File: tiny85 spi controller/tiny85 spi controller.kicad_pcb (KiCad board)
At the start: 2 copper layers, 11 parts, among them J1 rs232, J3 ISP, SW1 SW_Push, U1 MAX232, U2 ATtiny85V-10SU

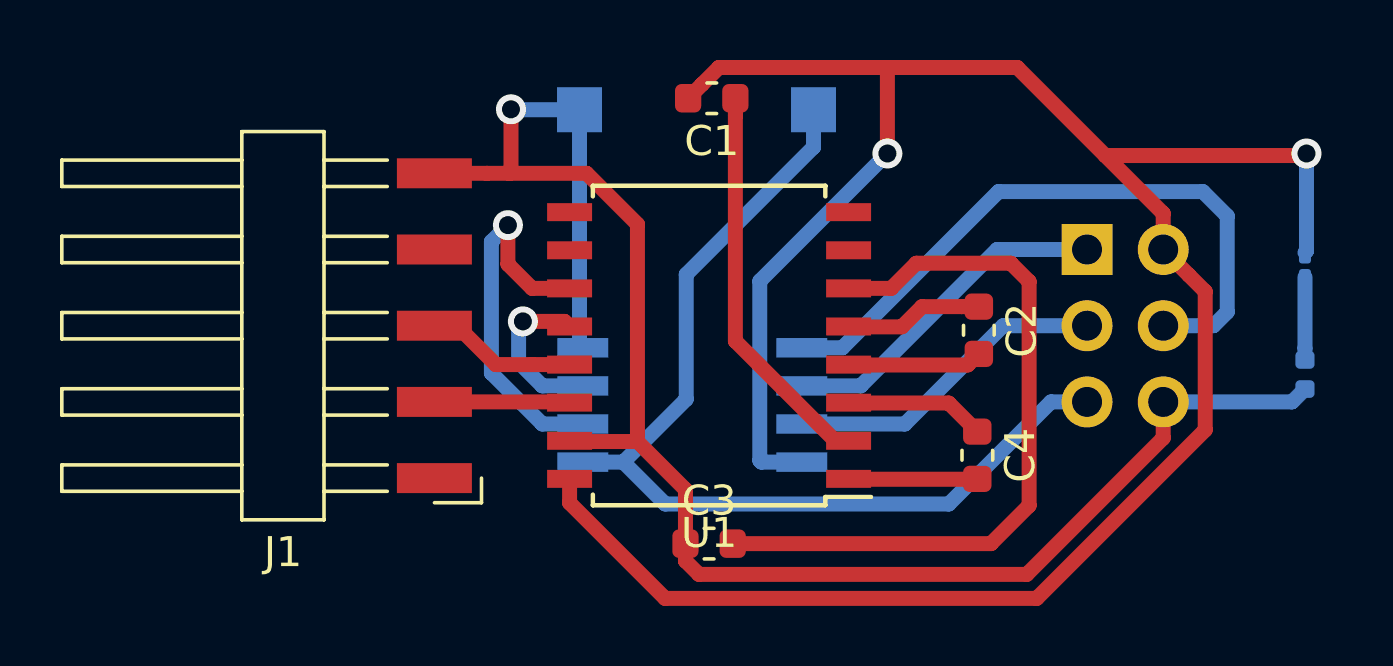
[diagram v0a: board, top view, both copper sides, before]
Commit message: some updates
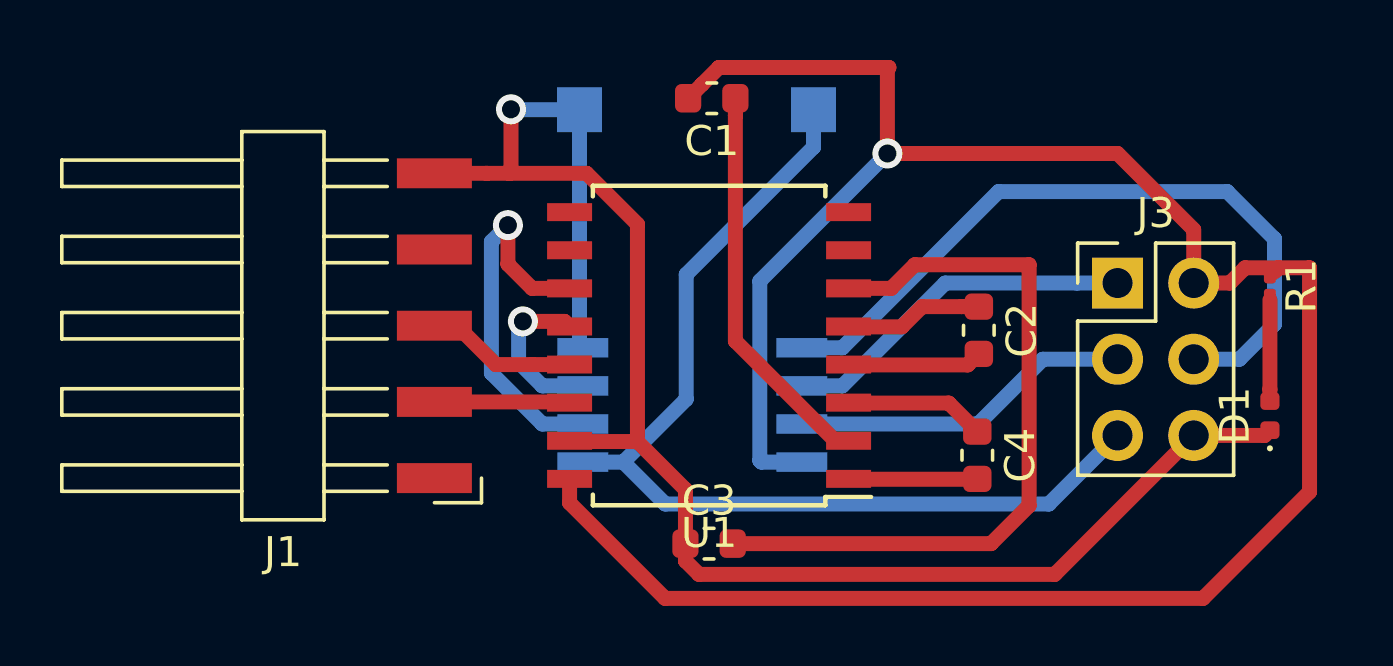
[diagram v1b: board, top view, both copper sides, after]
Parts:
- D1, R1: moved to F.Cu
- J3: footprint Connector_PinSocket_2.54mm:PinSocket_2x03_P2.54mm_Vertical -> Connector_PinHeader_2.54mm:PinHeader_2x03_P2.54mm_Vertical; moved to F.Cu
- moved D1 1.80 mm to (154.2, 56.0)
- moved J3 1.51 mm to (149.1, 51.6), turned to 0 degrees
- moved R1 1.34 mm to (154.2, 51.7)
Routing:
- net GND: track 58.2 -> 55.7 mm
- net Net-(J3-Pad4): track 22.2 -> 24.6 mm
- net Net-(C1-Pad2): track 78.1 -> 76.5 mm, vias 2 -> 1
- net Net-(D1-Pad2): track 2.76 -> 3.37 mm
- net Net-(J3-Pad3): track 10.9 -> 11.4 mm
- net Net-(J3-Pad1): track 11.4 -> 11.9 mm
- net Net-(J3-Pad5): track 33.2 -> 33.7 mm
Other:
- net class Default: via_drill 0.6 -> 0.5
